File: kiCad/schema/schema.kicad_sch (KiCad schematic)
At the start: 11 parts, among them J1 Esp32, J10 IR 4, J11 Switch, J2 DRV8833, J3 M1 Right, J4 M2 Left, J5 Bat, J6 Buck, J7 IR 1, J8 IR 3, J9 IR 2

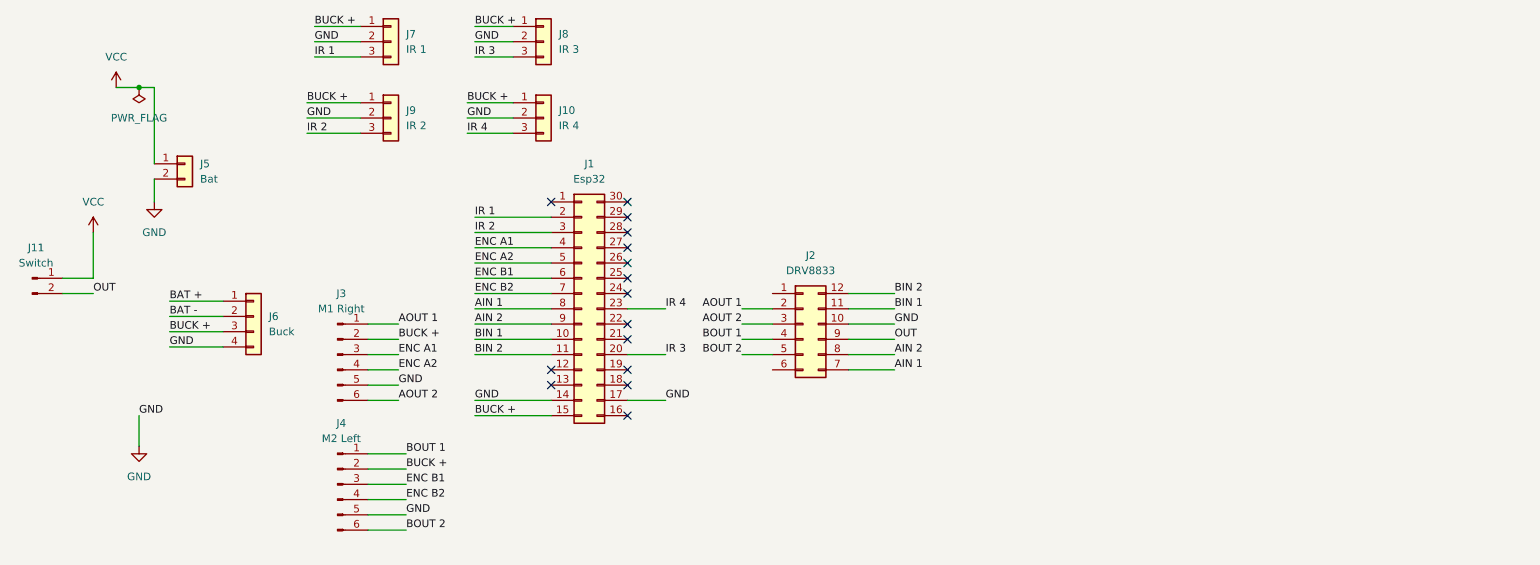
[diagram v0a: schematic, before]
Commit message: Day 7 - Schematics finished
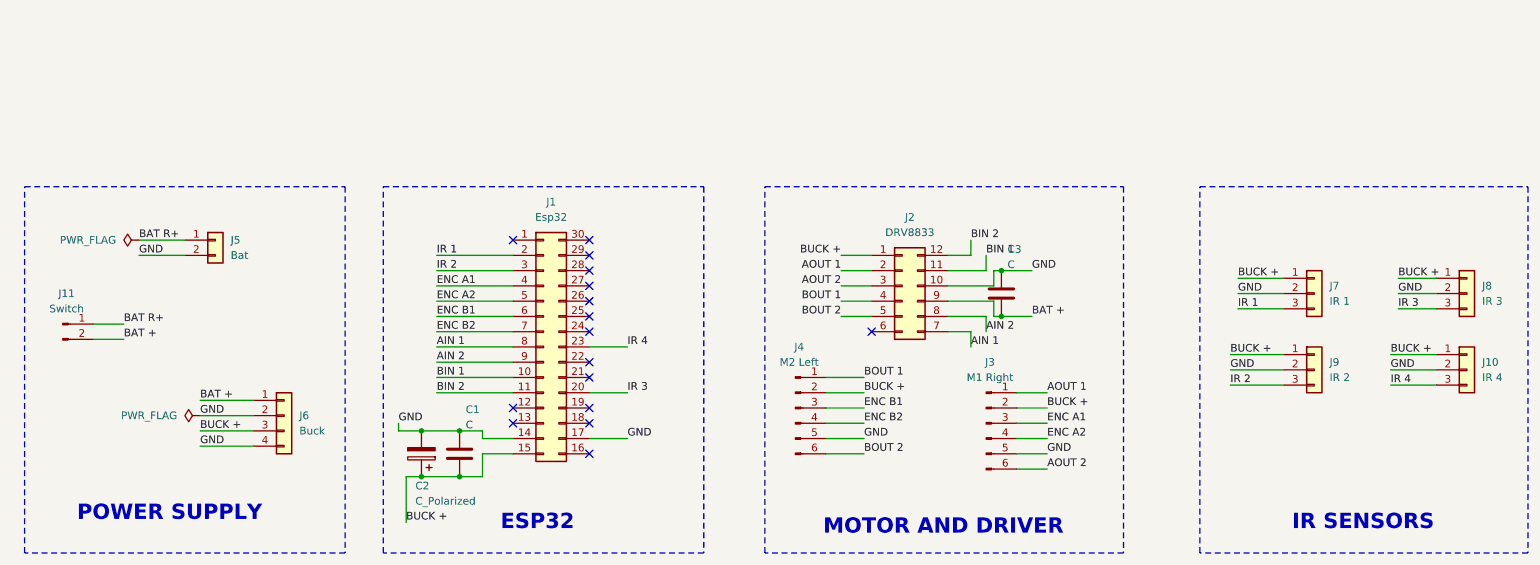
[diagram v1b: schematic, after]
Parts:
- added C1, C3: C, symbol Device:C
- added C2: C_Polarized, symbol Device:C_Polarized
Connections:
- net BAT - is gone; now on net GND: J6.2 (Pin_2)
- net OUT is gone; now on net BAT +: J11.2 (Pin_2), J2.9 (Pin_9)
- net BAT +: now also C3.2
- net BUCK +: now also J2.1 (Pin_1), C1.2, C2.1
- net GND: now also C1.1, C2.2, C3.1
- net VCC renamed BAT R+
- no-connect marks 15 -> 16
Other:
- note added: "ESP32"
- note added: "IR SENSORS"
- note added: "MOTOR AND DRIVER"
- note added: "POWER SUPPLY"
- moved on the sheet: J1, J10, J11, J2, J3, J4, J5, J6, J7, J8, J9
